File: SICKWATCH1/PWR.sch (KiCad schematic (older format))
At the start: 14 parts, among them J1 Conn_01x02_Female, U2 TLV71333PDBV, U3 MCP73831-2-OT, U4 74LVC1G17

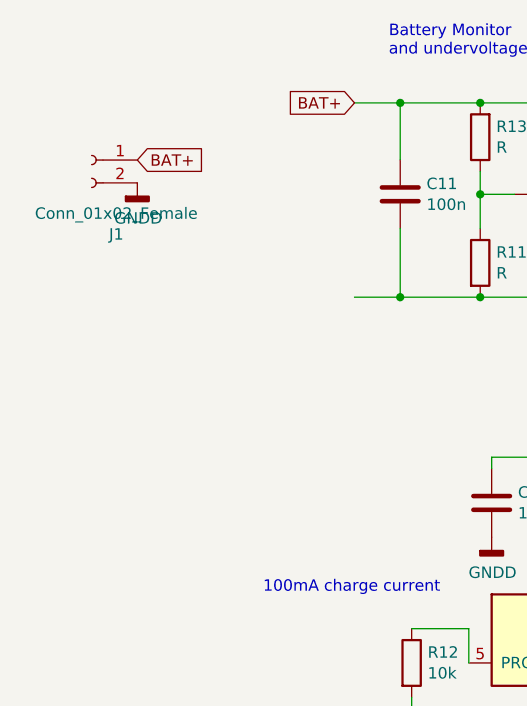
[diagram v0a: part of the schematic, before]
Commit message: Layout done (I GUESS)
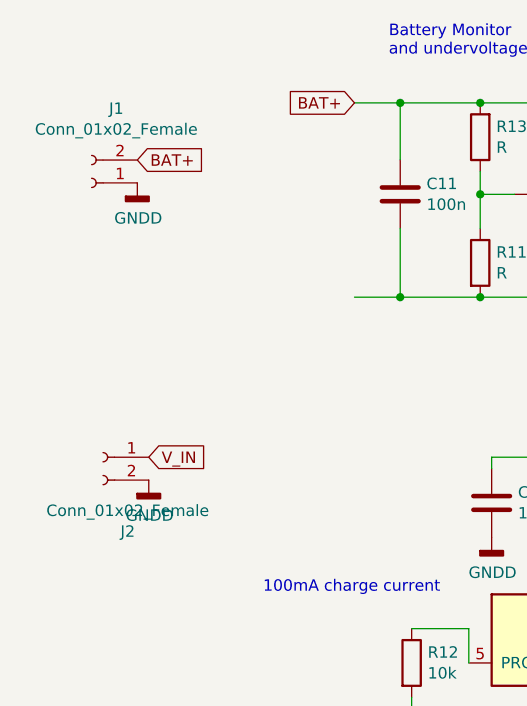
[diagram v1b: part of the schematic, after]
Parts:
- added J2: Conn_01x02_Female, Resistor_SMD:R_1206_3216Metric, symbol Connector:Conn_01x02_Female
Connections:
- net GND: now also J1.1 (Pin_1), J2.2 (Pin_2); no longer J1.2 (Pin_2)
- net VCC: now also J1.2 (Pin_2); no longer J1.1 (Pin_1)
- net V_IN: now also J2.1 (Pin_1)
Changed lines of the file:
@@
 L Connector:Conn_01x02_Female J1
 U 1 1 5DB313EC
-P 1600 2800
-F 0 "J1" H 1492 2475 50  0000 C CNN
-F 1 "Conn_01x02_Female" H 1492 2566 50  0000 C CNN
-F 2 "Connector_Molex:Molex_PicoBlade_53048-0210_1x02_P1.25mm_Horizontal" H 1600 2800 50  0001 C CNN
-F 3 "~" H 1600 2800 50  0001 C CNN
-	1    1600 2800
-	-1   0    0    -1
+P 1600 2900
+F 0 "J1" H 1492 2575 50  0000 C CNN
+F 1 "Conn_01x02_Female" H 1492 2666 50  0000 C CNN
+F 2 "Connector_Molex:Molex_PicoBlade_53048-0210_1x02_P1.25mm_Horizontal" H 1600 2900 50  0001 C CNN
+F 3 "~" H 1600 2900 50  0001 C CNN
+	1    1600 2900
+	-1   0    0    1
 $EndComp
 $Comp
@@
 	1    0    0    -1
 $EndComp
+$Comp
+L Connector:Conn_01x02_Female J2
+U 1 1 5DDA69D8
+P 1650 4100
+F 0 "J2" H 1542 3775 50  0000 C CNN
+F 1 "Conn_01x02_Female" H 1542 3866 50  0000 C CNN
+F 2 "Resistor_SMD:R_1206_3216Metric" H 1650 4100 50  0001 C CNN
+F 3 "~" H 1650 4100 50  0001 C CNN
+	1    1650 4100
+	-1   0    0    -1
+$EndComp
+$Comp
+L power:GNDD #PWR0105
+U 1 1 5DDA69DE
+P 1850 4200
+F 0 "#PWR0105" H 1850 3950 50  0001 C CNN
+F 1 "GNDD" H 1854 4045 50  0000 C CNN
+F 2 "" H 1850 4200 50  0001 C CNN
+F 3 "" H 1850 4200 50  0001 C CNN
+	1    1850 4200
+	1    0    0    -1
+$EndComp
+Text GLabel 1850 4100 2    50   Input ~ 0
+V_IN
 $EndSCHEMATC
